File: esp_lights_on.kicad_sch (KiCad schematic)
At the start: 19 parts, among them J2 Conn_01x06_Pin, J3 VIN, J4 Screw_Terminal_01x03, K1 RELAY, K2 RELAY, Q1 SS8050, Q2 SS8050, U1 ESP32-WROOM-32, U2 TLV1117-33

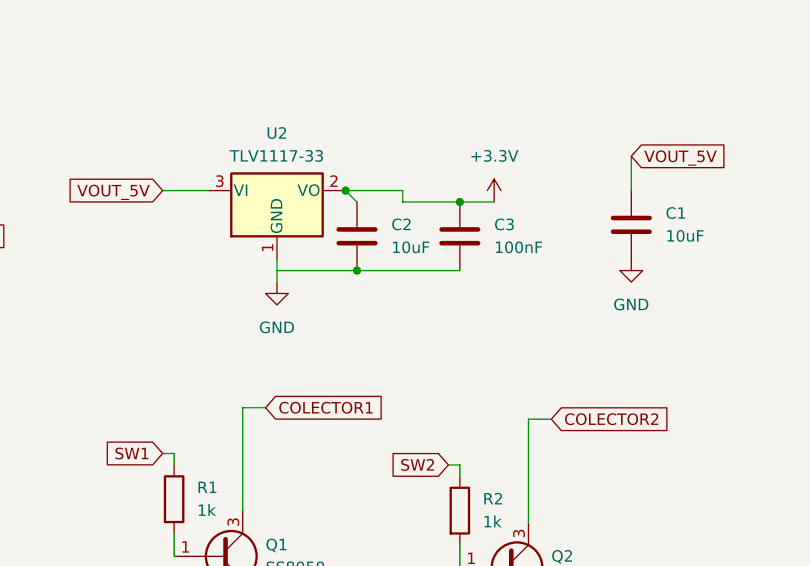
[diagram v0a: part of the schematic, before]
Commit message: final commit
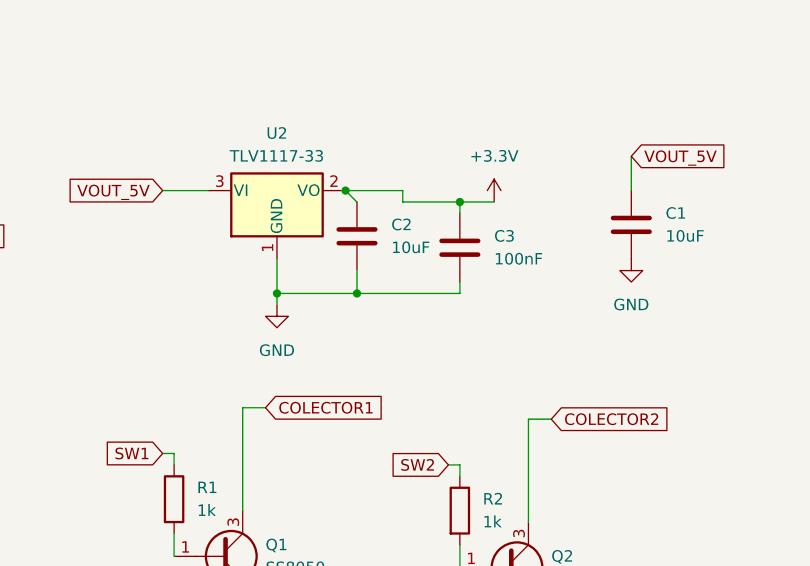
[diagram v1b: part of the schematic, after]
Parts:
- R1, R2: footprint Resistor_SMD:R_1206_3216Metric_Pad1.30x1.75mm_HandSolder -> Resistor_SMD:R_0805_2012Metric
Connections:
- net GND: now also C2.2, C3.2
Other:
- moved on the sheet: C3
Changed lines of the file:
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@@
 	)
 	(junction
-		(at 173.99 96.52)
+		(at 106.68 45.72)
 		(diameter 0)
 		(color 0 0 0 0)
 	)
 	(junction
-		(at 127 35.56)
+		(at 173.99 96.52)
 		(diameter 0)
 		(color 0 0 0 0)
@@
 	)
 	(junction
+		(at 115.57 45.72)
+		(diameter 0)
+		(color 0 0 0 0)
+	)
+	(junction
 		(at 250.19 96.52)
 		(diameter 0)
@@
 	)
 	(junction
-		(at 115.57 43.18)
+		(at 127 35.56)
 		(diameter 0)
 		(color 0 0 0 0)
@@
 	(wire
 		(pts
-			(xy 106.68 43.18) (xy 115.57 43.18)
+			(xy 106.68 45.72) (xy 115.57 45.72)
 		)
 		(stroke
@@
 	(wire
 		(pts
+			(xy 115.57 45.72) (xy 127 45.72)
+		)
+		(stroke
+			(width 0)
+			(type default)
+		)
+	)
+	(wire
+		(pts
 			(xy 95.25 63.5) (xy 95.25 64.77)
 		)
@@
 	(wire
 		(pts
+			(xy 127 36.83) (xy 127 35.56)
+		)
+		(stroke
+			(width 0)
+			(type default)
+		)
+	)
+	(wire
+		(pts
 			(xy 173.99 96.52) (xy 177.8 96.52)
 		)
@@
 	(wire
 		(pts
-			(xy 182.88 114.3) (xy 182.88 111.76)
+			(xy 115.57 45.72) (xy 115.57 43.18)
 		)
 		(stroke
@@
 	(wire
 		(pts
-			(xy 83.82 142.24) (xy 88.9 142.24)
+			(xy 182.88 114.3) (xy 182.88 111.76)
 		)
 		(stroke
@@
 	(wire
 		(pts
-			(xy 93.98 34.29) (xy 99.06 34.29)
+			(xy 83.82 142.24) (xy 88.9 142.24)
 		)
 		(stroke
@@
 	(wire
 		(pts
-			(xy 252.73 96.52) (xy 252.73 97.79)
+			(xy 93.98 34.29) (xy 99.06 34.29)
 		)
 		(stroke
@@
 	(wire
 		(pts
-			(xy 102.87 58.42) (xy 102.87 69.85)
+			(xy 252.73 96.52) (xy 252.73 97.79)
 		)
 		(stroke
@@
 	(wire
 		(pts
-			(xy 220.98 78.74) (xy 218.44 78.74)
+			(xy 102.87 58.42) (xy 102.87 69.85)
 		)
 		(stroke
@@
 	(wire
 		(pts
-			(xy 115.57 43.18) (xy 127 43.18)
+			(xy 220.98 78.74) (xy 218.44 78.74)
 		)
 		(stroke
@@
 	(wire
 		(pts
+			(xy 106.68 45.72) (xy 106.68 46.99)
+		)
+		(stroke
+			(width 0)
+			(type default)
+		)
+	)
+	(wire
+		(pts
 			(xy 250.19 116.84) (xy 250.19 96.52)
 		)
@@
 	(wire
 		(pts
+			(xy 106.68 41.91) (xy 106.68 45.72)
+		)
+		(stroke
+			(width 0)
+			(type default)
+		)
+	)
+	(wire
+		(pts
 			(xy 146.05 30.48) (xy 146.05 34.29)
 		)
@@
 	(wire
 		(pts
-			(xy 120.65 34.29) (xy 114.3 34.29)
+			(xy 127 45.72) (xy 127 44.45)
 		)
 		(stroke
@@
 	(wire
 		(pts
-			(xy 104.14 119.38) (xy 104.14 132.08)
+			(xy 120.65 34.29) (xy 114.3 34.29)
 		)
 		(stroke
@@
 	(wire
 		(pts
-			(xy 100.33 119.38) (xy 104.14 119.38)
+			(xy 104.14 119.38) (xy 104.14 132.08)
 		)
 		(stroke
@@
 	(wire
 		(pts
-			(xy 106.68 41.91) (xy 106.68 44.45)
+			(xy 100.33 119.38) (xy 104.14 119.38)
 		)
 		(stroke
@@
 			)
 		)
-		(property "Footprint" "Resistor_SMD:R_1206_3216Metric_Pad1.30x1.75mm_HandSolder"
+		(property "Footprint" "Resistor_SMD:R_0805_2012Metric"
 			(at 93.472 68.58 90)
 			(hide yes)
@@
 	(symbol
 		(lib_id "Device:C")
-		(at 127 39.37 0)
+		(at 127 40.64 0)
 		(unit 1)
 		(body_style 1)
@@
 		(fields_autoplaced yes)
 		(property "Reference" "C3"
-			(at 130.81 38.0999 0)
+			(at 130.81 39.3699 0)
 			(show_name no)
 			(do_not_autoplace no)
@@
 		)
 		(property "Value" "100nF"
-			(at 130.81 40.6399 0)
+			(at 130.81 41.9099 0)
 			(show_name no)
 			(do_not_autoplace no)
@@
 		)
 		(property "Footprint" "Capacitor_SMD:C_0805_2012Metric_Pad1.18x1.45mm_HandSolder"
-			(at 127.9652 43.18 0)
+			(at 127.9652 44.45 0)
 			(hide yes)
 			(show_name no)
@@
 		)
 		(property "Datasheet" ""
-			(at 127 39.37 0)
+			(at 127 40.64 0)
 			(hide yes)
 			(show_name no)
@@
 		)
 		(property "Description" "Unpolarized capacitor"
-			(at 127 39.37 0)
+			(at 127 40.64 0)
 			(hide yes)
 			(show_name no)
@@
 	(symbol
 		(lib_id "power:GND")
-		(at 106.68 44.45 0)
+		(at 106.68 46.99 0)
 		(unit 1)
 		(body_style 1)
@@
 		(fields_autoplaced yes)
 		(property "Reference" "#PWR01"
-			(at 106.68 50.8 0)
+			(at 106.68 53.34 0)
 			(hide yes)
 			(show_name no)
@@
 		)
 		(property "Value" "GND"
-			(at 106.68 49.53 0)
+			(at 106.68 52.07 0)
 			(show_name no)
 			(do_not_autoplace no)
@@
 		)
 		(property "Footprint" ""
-			(at 106.68 44.45 0)
+			(at 106.68 46.99 0)
 			(hide yes)
 			(show_name no)
@@
 		)
 		(property "Datasheet" ""
-			(at 106.68 44.45 0)
+			(at 106.68 46.99 0)
 			(hide yes)
 			(show_name no)
@@
 		)
 		(property "Description" "Power symbol creates a global label with name \"GND\" , ground"
-			(at 106.68 44.45 0)
+			(at 106.68 46.99 0)
 			(hide yes)
 			(show_name no)
@@
 			)
 		)
-		(property "Footprint" "Resistor_SMD:R_1206_3216Metric_Pad1.30x1.75mm_HandSolder"
+		(property "Footprint" "Resistor_SMD:R_0805_2012Metric"
 			(at 125.222 69.85 90)
 			(hide yes)

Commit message: modifications by ovi
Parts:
- K1, K2: footprint Relay_THT:Relay_SPST_Panasonic_ADW11 -> RELAYs:0JT-SS-105LM
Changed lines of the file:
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@@
 			)
 		)
-		(property "Footprint" "Relay_THT:Relay_SPST_Panasonic_ADW11"
+		(property "Footprint" "RELAYs:0JT-SS-105LM"
 			(at 45.72 146.05 0)
 			(hide yes)
@@
 			)
 		)
-		(property "Footprint" "Relay_THT:Relay_SPST_Panasonic_ADW11"
+		(property "Footprint" "RELAYs:0JT-SS-105LM"
 			(at 95.25 148.59 0)
 			(hide yes)
